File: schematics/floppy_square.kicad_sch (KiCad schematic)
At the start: 6 parts, among them J1 Conn_01x07_Pin, SW1 SW_Push, SW2 SW_Push, U1 D168K, U2 D168K

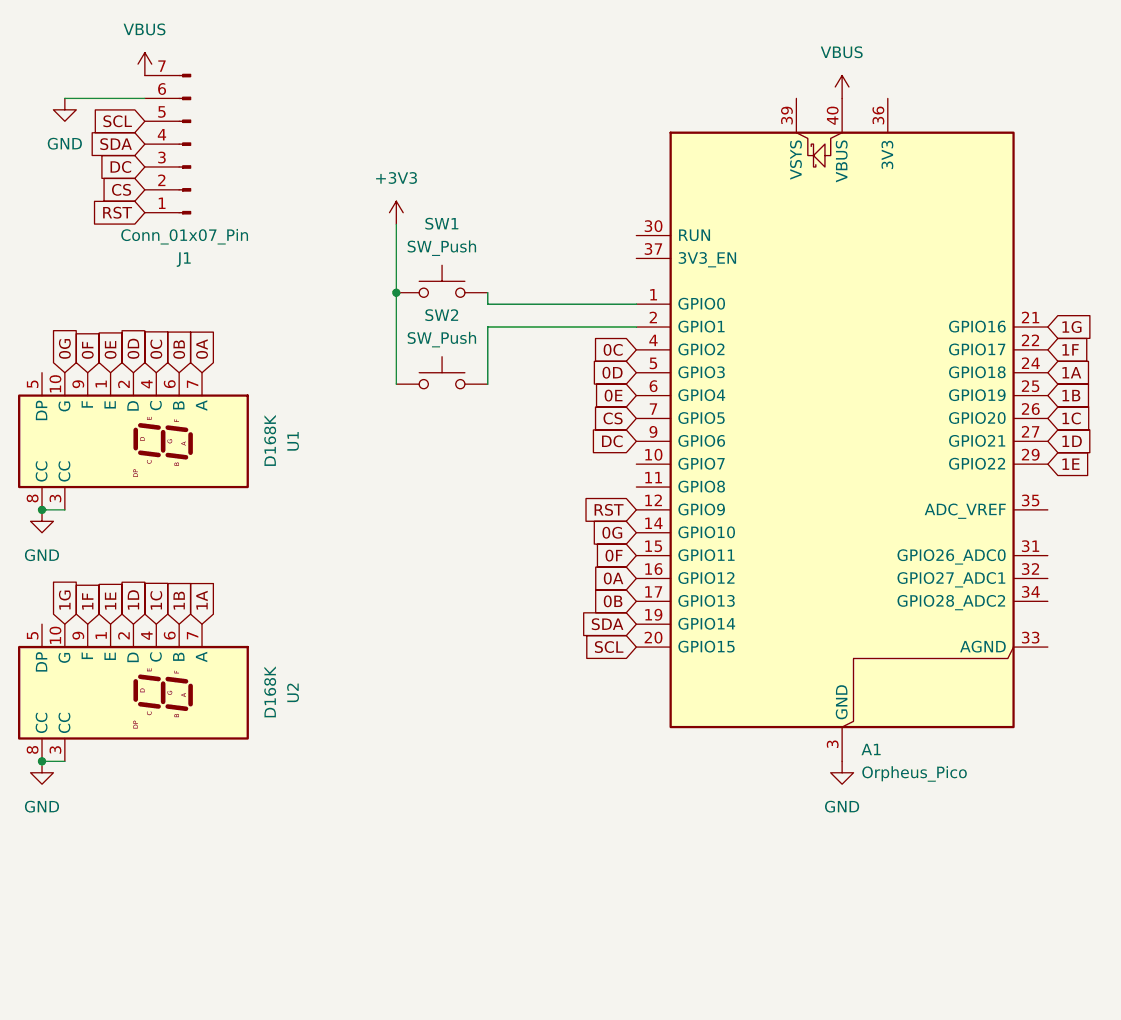
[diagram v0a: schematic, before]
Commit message: feat: A buncha stuff
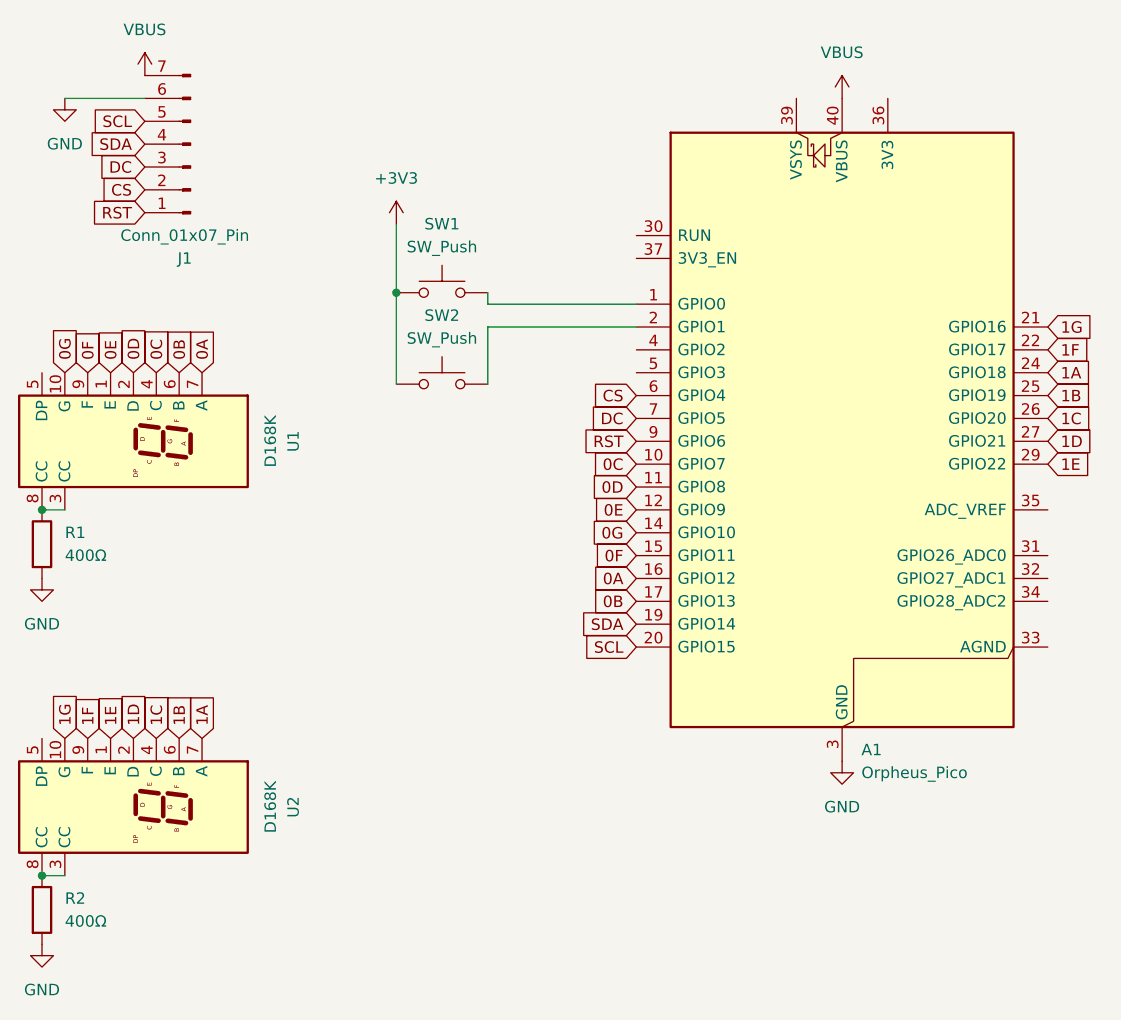
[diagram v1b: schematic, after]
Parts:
- added R1, R2: 400Ω, symbol Device:R
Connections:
- net 0C: now also A1.10 (GPIO7); no longer A1.4 (GPIO2)
- net 0D: now also A1.11 (GPIO8); no longer A1.5 (GPIO3)
- net 0E: now also A1.12 (GPIO9); no longer A1.6 (GPIO4)
- net CS: now also A1.6 (GPIO4); no longer A1.7 (GPIO5)
- net DC: now also A1.7 (GPIO5); no longer A1.9 (GPIO6)
- net GND: now also R1.2, R2.2; no longer U1.3 (CC), U1.8 (CC), U2.3 (CC), U2.8 (CC)
- net RST: now also A1.9 (GPIO6); no longer A1.12 (GPIO9)
- new net: R1.1, U1.3 (CC), U1.8 (CC)
- new net: R2.1, U2.3 (CC), U2.8 (CC)
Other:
- moved on the sheet: U2
